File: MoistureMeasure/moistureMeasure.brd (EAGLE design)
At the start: 49.5 x 32.4 mm, 8 parts, among them IC1 74HC14D, Q1 BC847BSMD

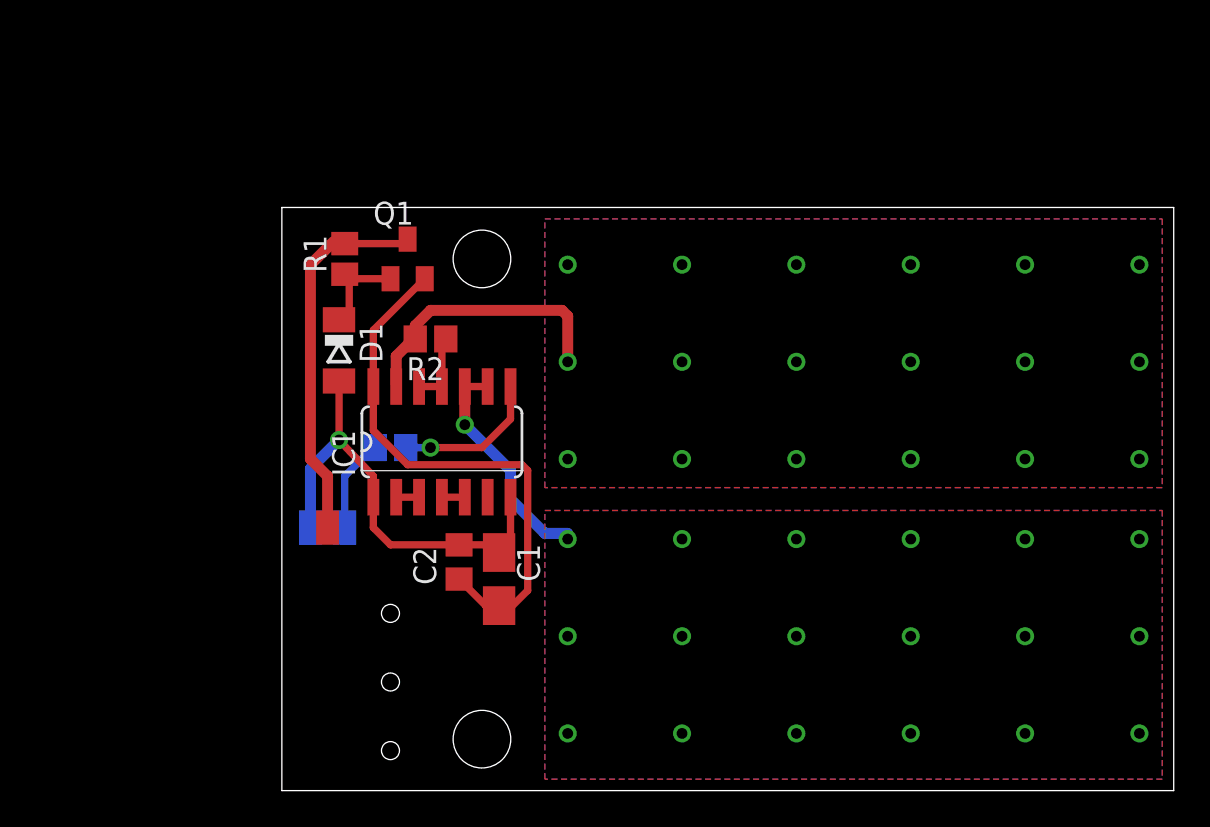
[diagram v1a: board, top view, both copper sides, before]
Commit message: mainBoard update
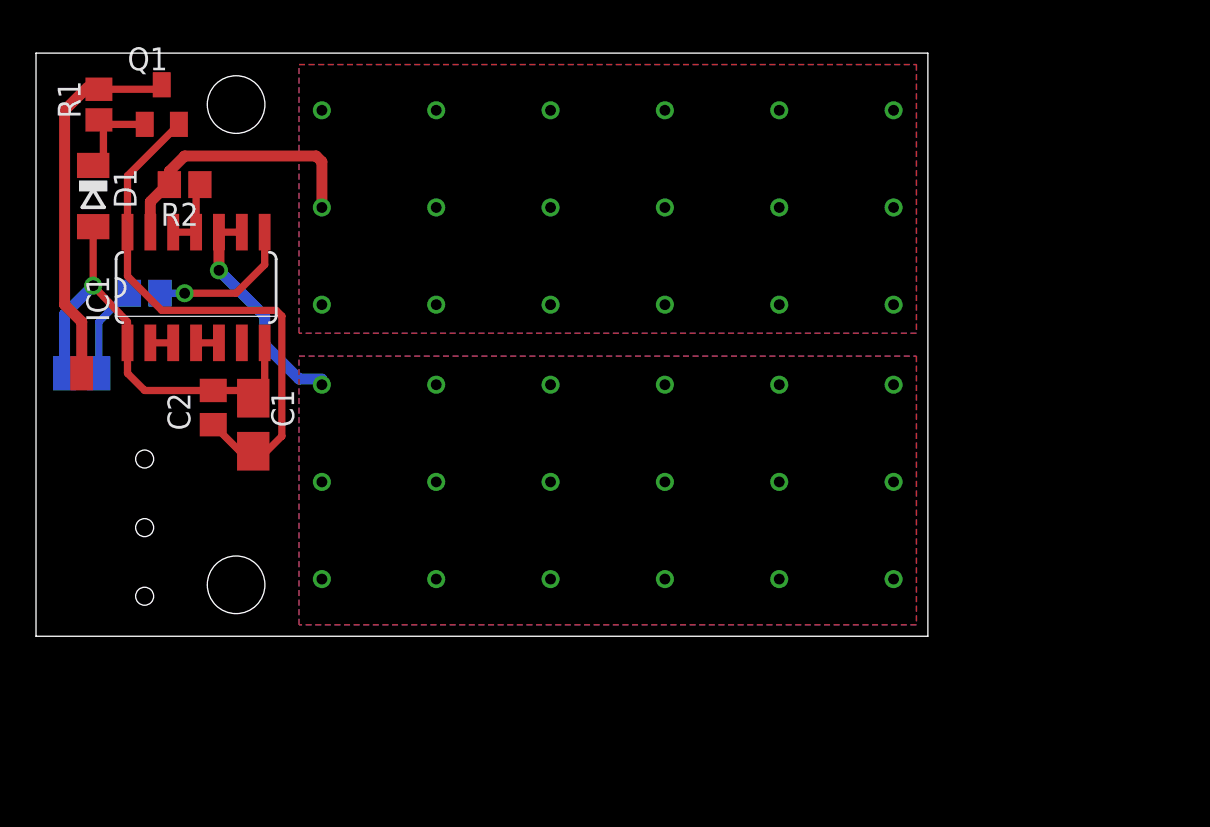
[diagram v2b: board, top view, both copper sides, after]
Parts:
- moved C1 16.1 mm to (12.1, 11.7)
- moved C2 16.1 mm to (9.84, 12.7)
- moved D1 16.1 mm to (3.17, 24.4)
- moved Q1 16.1 mm to (6.99, 29.5)
- moved R1 16.1 mm to (3.49, 29.5)
- moved R3 16.1 mm to (6.03, 19.1)
- moved IC1 16.1 mm to (8.89, 19.4)
- moved R2 16.1 mm to (8.26, 25.1)
